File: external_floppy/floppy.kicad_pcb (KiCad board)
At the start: 2 copper layers, 96.5 x 44.5 mm, 13 parts, among them J1 12VDC, J2 FLOPPY_PWR, J3 ADAPTER, J4 FLOPPY, SW1 SW_DPDT_x2, U1 L7805

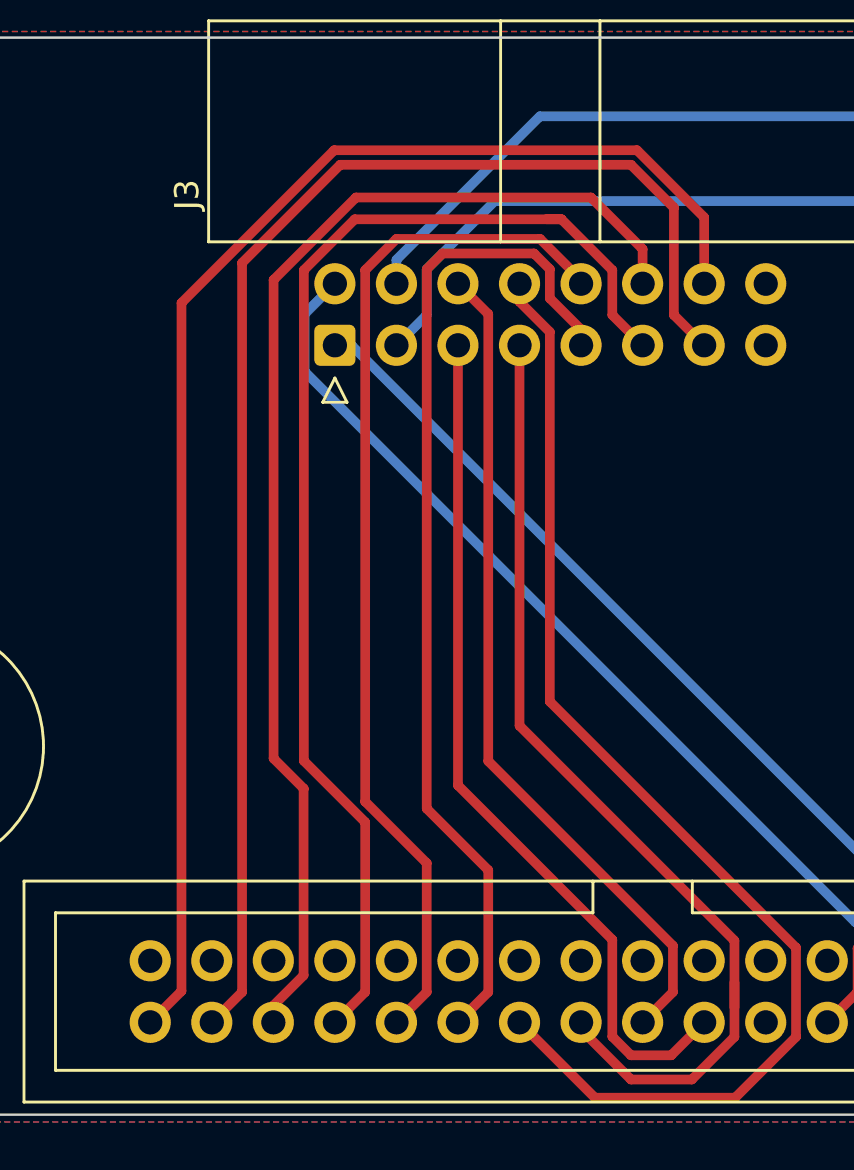
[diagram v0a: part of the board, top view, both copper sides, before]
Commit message: a
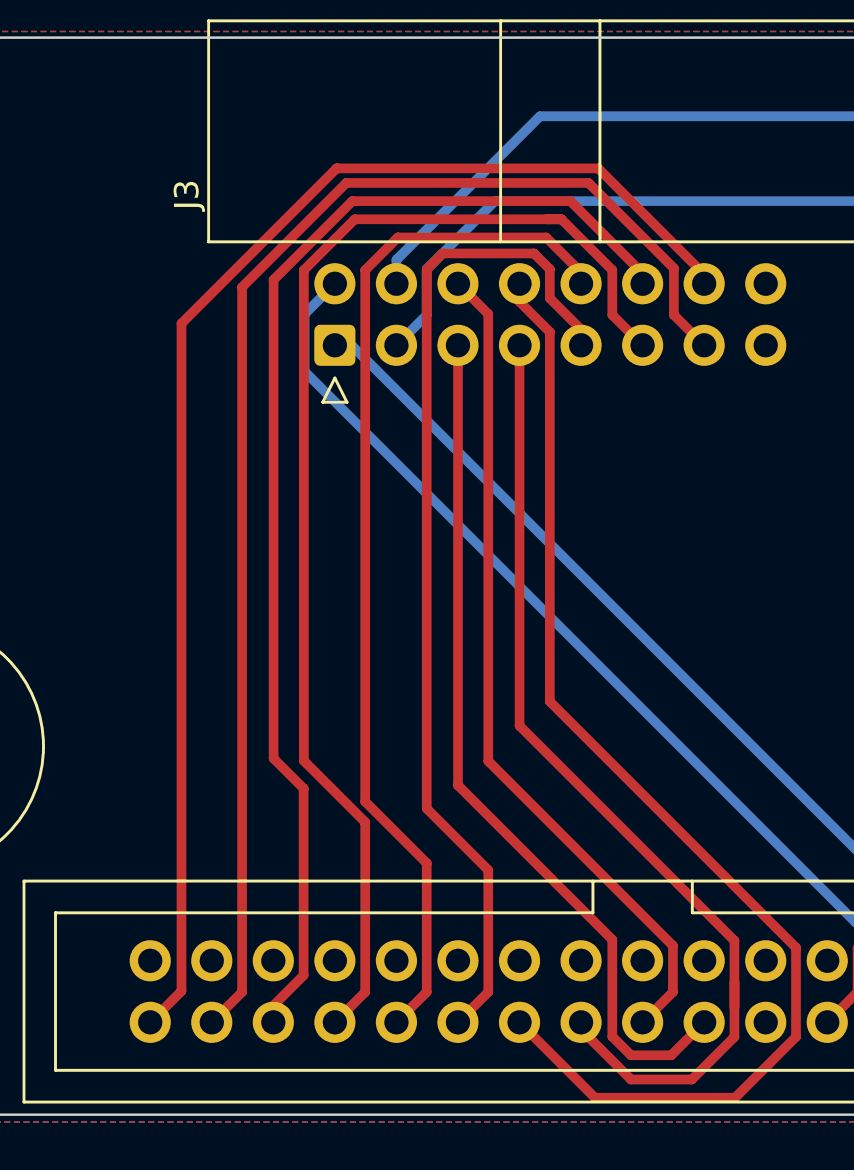
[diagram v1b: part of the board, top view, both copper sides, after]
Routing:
- net /FLOPPY_SIDE_SELECT: track 58.3 -> 55.6 mm
- net /FLOPPY_READY: track 58.9 -> 56.5 mm
- net /FLOPPY_READ_DATA: track 50.6 -> 49.9 mm
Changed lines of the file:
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@@
   (segment (start 51.435 95.885) (end 55.245 95.885) (width 0.4) (layer "F.Cu") (net 3))
   (segment (start 55.245 76.835) (end 55.245 81.915) (width 0.4) (layer "F.Cu") (net 4))
-  (segment (start 81.251467 68.149991) (end 74.949999 74.451459) (width 0.4) (layer "F.Cu") (net 5))
+  (segment (start 81.35001 68.89999) (end 81.425739 68.89999) (width 0.4) (layer "F.Cu") (net 5))
+  (segment (start 81.35001 68.89999) (end 92.14999 68.89999) (width 0.4) (layer "F.Cu") (net 5))
   (segment (start 96.52 73.02) (end 96.52 73.66) (width 0.4) (layer "F.Cu") (net 5))
-  (segment (start 96.52 73.66) (end 96.52 70.921458) (width 0.4) (layer "F.Cu") (net 5))
-  (segment (start 93.748532 68.14999) (end 81.251467 68.149991) (width 0.4) (layer "F.Cu") (net 5))
-  (segment (start 74.949999 74.451459) (end 74.949999 102.850001) (width 0.4) (layer "F.Cu") (net 5))
-  (segment (start 96.52 70.921458) (end 93.748532 68.14999) (width 0.4) (layer "F.Cu") (net 5))
-  (segment (start 74.949999 102.850001) (end 73.66 104.14) (width 0.4) (layer "F.Cu") (net 5))
+  (segment (start 74.949999 102.850001) (end 74.949999 75.300001) (width 0.4) (layer "F.Cu") (net 5))
+  (segment (start 73.66 104.14) (end 74.949999 102.850001) (width 0.4) (layer "F.Cu") (net 5))
+  (segment (start 74.949999 75.300001) (end 81.35001 68.89999) (width 0.4) (layer "F.Cu") (net 5))
+  (segment (start 92.14999 68.89999) (end 96.52 73.27) (width 0.4) (layer "F.Cu") (net 5))
+  (segment (start 96.52 73.27) (end 96.52 73.66) (width 0.4) (layer "F.Cu") (net 5))
   (segment (start 78.74 104.14) (end 78.74 103.450002) (width 0.4) (layer "F.Cu") (net 6))
-  (segment (start 91.85001 70.10001) (end 82.14999 70.10001) (width 0.4) (layer "F.Cu") (net 6))
-  (segment (start 93.98 73.66) (end 93.98 72.23) (width 0.4) (layer "F.Cu") (net 6))
+  (segment (start 93.98 73.66) (end 93.98 73.23) (width 0.4) (layer "F.Cu") (net 6))
+  (segment (start 93.98 73.23) (end 91 70.25) (width 0.4) (layer "F.Cu") (net 6))
+  (segment (start 82 70.25) (end 78.75 73.5) (width 0.4) (layer "F.Cu") (net 6))
+  (segment (start 78.75 73.5) (end 78.75 93.25) (width 0.4) (layer "F.Cu") (net 6))
   (segment (start 79.990001 102.200001) (end 79.990001 94.490001) (width 0.4) (layer "F.Cu") (net 6))
+  (segment (start 78.75 93.25) (end 80 94.5) (width 0.4) (layer "F.Cu") (net 6))
+  (segment (start 91 70.25) (end 82 70.25) (width 0.4) (layer "F.Cu") (net 6))
   (segment (start 78.74 103.450002) (end 79.990001 102.200001) (width 0.4) (layer "F.Cu") (net 6))
-  (segment (start 82.14999 70.10001) (end 78.75 73.5) (width 0.4) (layer "F.Cu") (net 6))
-  (segment (start 78.75 93.25) (end 80 94.5) (width 0.4) (layer "F.Cu") (net 6))
-  (segment (start 93.98 72.23) (end 91.85001 70.10001) (width 0.4) (layer "F.Cu") (net 6))
-  (segment (start 78.75 73.5) (end 78.75 93.25) (width 0.4) (layer "F.Cu") (net 6))
-  (segment (start 89.748534 71.80999) (end 91.44 73.501456) (width 0.4) (layer "F.Cu") (net 7))
-  (segment (start 85.070001 102.889999) (end 85.070001 97.570001) (width 0.4) (layer "F.Cu") (net 7))
-  (segment (start 82.530001 73.099997) (end 83.820009 71.809989) (width 0.4) (layer "F.Cu") (net 7))
-  (segment (start 82.530001 95.030001) (end 82.530001 73.099997) (width 0.4) (layer "F.Cu") (net 7))
-  (segment (start 91.44 73.501456) (end 91.44 73.66) (width 0.4) (layer "F.Cu") (net 7))
-  (segment (start 83.820009 71.809989) (end 89.748534 71.80999) (width 0.4) (layer "F.Cu") (net 7))
-  (segment (start 85.070001 97.570001) (end 82.530001 95.030001) (width 0.4) (layer "F.Cu") (net 7))
-  (segment (start 83.82 104.14) (end 85.070001 102.889999) (width 0.4) (layer "F.Cu") (net 7))
+  (segment (start 85.070001 102.889999) (end 83.82 104.14) (width 0.4) (layer "F.Cu") (net 7))
+  (segment (start 83.879998 71.75) (end 83.820009 71.809989) (width 0.4) (layer "F.Cu") (net 7))
+  (segment (start 90 71.75) (end 83.879998 71.75) (width 0.4) (layer "F.Cu") (net 7))
+  (segment (start 91.44 73.19) (end 90 71.75) (width 0.4) (layer "F.Cu") (net 7))
+  (segment (start 85.070001 97.570001) (end 85.070001 102.889999) (width 0.4) (layer "F.Cu") (net 7))
+  (segment (start 82.530001 73.099997) (end 82.530001 95.030001) (width 0.4) (layer "F.Cu") (net 7))
+  (segment (start 83.879998 71.75) (end 82.530001 73.099997) (width 0.4) (layer "F.Cu") (net 7))
+  (segment (start 82.530001 95.030001) (end 85.070001 97.570001) (width 0.4) (layer "F.Cu") (net 7))
+  (segment (start 91.44 73.66) (end 91.44 73.19) (width 0.4) (layer "F.Cu") (net 7))
   (segment (start 100.310001 101.060001) (end 100.310001 104.740001) (width 0.4) (layer "F.Cu") (net 8))
   (segment (start 97.800002 107.25) (end 92.01 107.25) (width 0.4) (layer "F.Cu") (net 8))
@@
   (segment (start 80.02999 77.27999) (end 102.75 100) (width 0.4) (layer "B.Cu") (net 11))
   (segment (start 80.02999 74.91001) (end 80.02999 77.27999) (width 0.4) (layer "B.Cu") (net 11))
-  (segment (start 77.450001 72.799999) (end 81.5 68.75) (width 0.4) (layer "F.Cu") (net 12))
-  (segment (start 77.450001 102.889999) (end 77.450001 72.799999) (width 0.4) (layer "F.Cu") (net 12))
-  (segment (start 95.269999 70.519999) (end 95.269999 74.949999) (width 0.4) (layer "F.Cu") (net 12))
-  (segment (start 81.5 68.75) (end 93.5 68.75) (width 0.4) (layer "F.Cu") (net 12))
-  (segment (start 93.5 68.75) (end 95.269999 70.519999) (width 0.4) (layer "F.Cu") (net 12))
+  (segment (start 91.75 69.5) (end 95.269999 73.019999) (width 0.4) (layer "F.Cu") (net 12))
+  (segment (start 77.450001 102.889999) (end 77.450001 73.799999) (width 0.4) (layer "F.Cu") (net 12))
+  (segment (start 81.75 69.5) (end 91.75 69.5) (width 0.4) (layer "F.Cu") (net 12))
+  (segment (start 77.450001 73.799999) (end 81.75 69.5) (width 0.4) (layer "F.Cu") (net 12))
   (segment (start 95.269999 74.949999) (end 96.52 76.2) (width 0.4) (layer "F.Cu") (net 12))
   (segment (start 76.2 104.14) (end 77.450001 102.889999) (width 0.4) (layer "F.Cu") (net 12))
+  (segment (start 95.269999 73.019999) (end 95.269999 74.949999) (width 0.4) (layer "F.Cu") (net 12))
+  (segment (start 82.530001 102.889999) (end 81.28 104.14) (width 0.4) (layer "F.Cu") (net 13))
+  (segment (start 82.098542 71) (end 80 73.098542) (width 0.4) (layer "F.Cu") (net 13))
+  (segment (start 90.630002 71) (end 82.098542 71) (width 0.4) (layer "F.Cu") (net 13))
   (segment (start 93.98 76.2) (end 92.729999 74.949999) (width 0.4) (layer "F.Cu") (net 13))
-  (segment (start 90.630002 71) (end 82.098542 71) (width 0.4) (layer "F.Cu") (net 13))
+  (segment (start 82.530001 95.878543) (end 82.530001 102.889999) (width 0.4) (layer "F.Cu") (net 13))
   (segment (start 92.729999 74.949999) (end 92.729999 73.099997) (width 0.4) (layer "F.Cu") (net 13))
-  (segment (start 82.530001 102.889999) (end 81.28 104.14) (width 0.4) (layer "F.Cu") (net 13))
-  (segment (start 82.530001 95.878543) (end 82.530001 102.889999) (width 0.4) (layer "F.Cu") (net 13))
   (segment (start 92.729999 73.099997) (end 90.630002 71) (width 0.4) (layer "F.Cu") (net 13))
   (segment (start 90.630002 71) (end 90 71) (width 0.4) (layer "F.Cu") (net 13))
+  (segment (start 80 93.348542) (end 82.530001 95.878543) (width 0.4) (layer "F.Cu") (net 13))
   (segment (start 80 73.098542) (end 80 93.348542) (width 0.4) (layer "F.Cu") (net 13))
-  (segment (start 82.098542 71) (end 80 73.098542) (width 0.4) (layer "F.Cu") (net 13))
-  (segment (start 80 93.348542) (end 82.530001 95.878543) (width 0.4) (layer "F.Cu") (net 13))
   (segment (start 90.150001 74.260001) (end 90.150001 73.059999) (width 0.4) (layer "F.Cu") (net 14))
   (segment (start 91.44 76.2) (end 91.44 75.55) (width 0.4) (layer "F.Cu") (net 14))
